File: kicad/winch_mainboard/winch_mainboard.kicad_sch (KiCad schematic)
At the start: 35 parts, among them J1 PWR_IN_24V (from Victron 96V-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, J10 Heltec WiFi LoRa 32 V4 - Head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, J11 Heltec WiFi LoRa 32 V4 - Head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, J12 Hall sensors (drum direction), J2 CAN_BUS (to Fardriver), J3 To GIGA UART (TXD,RXD,GND), J4 HX711 module (3V3,GND,DT,SCK), J6 Spare I/O, J7 Line cut switch (winch), J8 Winchman remote switches, J9 Cut motor out (24V) - A/B = K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, K1 Relay 24V coil (Songle SRD-24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, Q1 BC337-40, U1 ESP32-S3 N16R8 DevKitC-1, U3 SN65HVD230

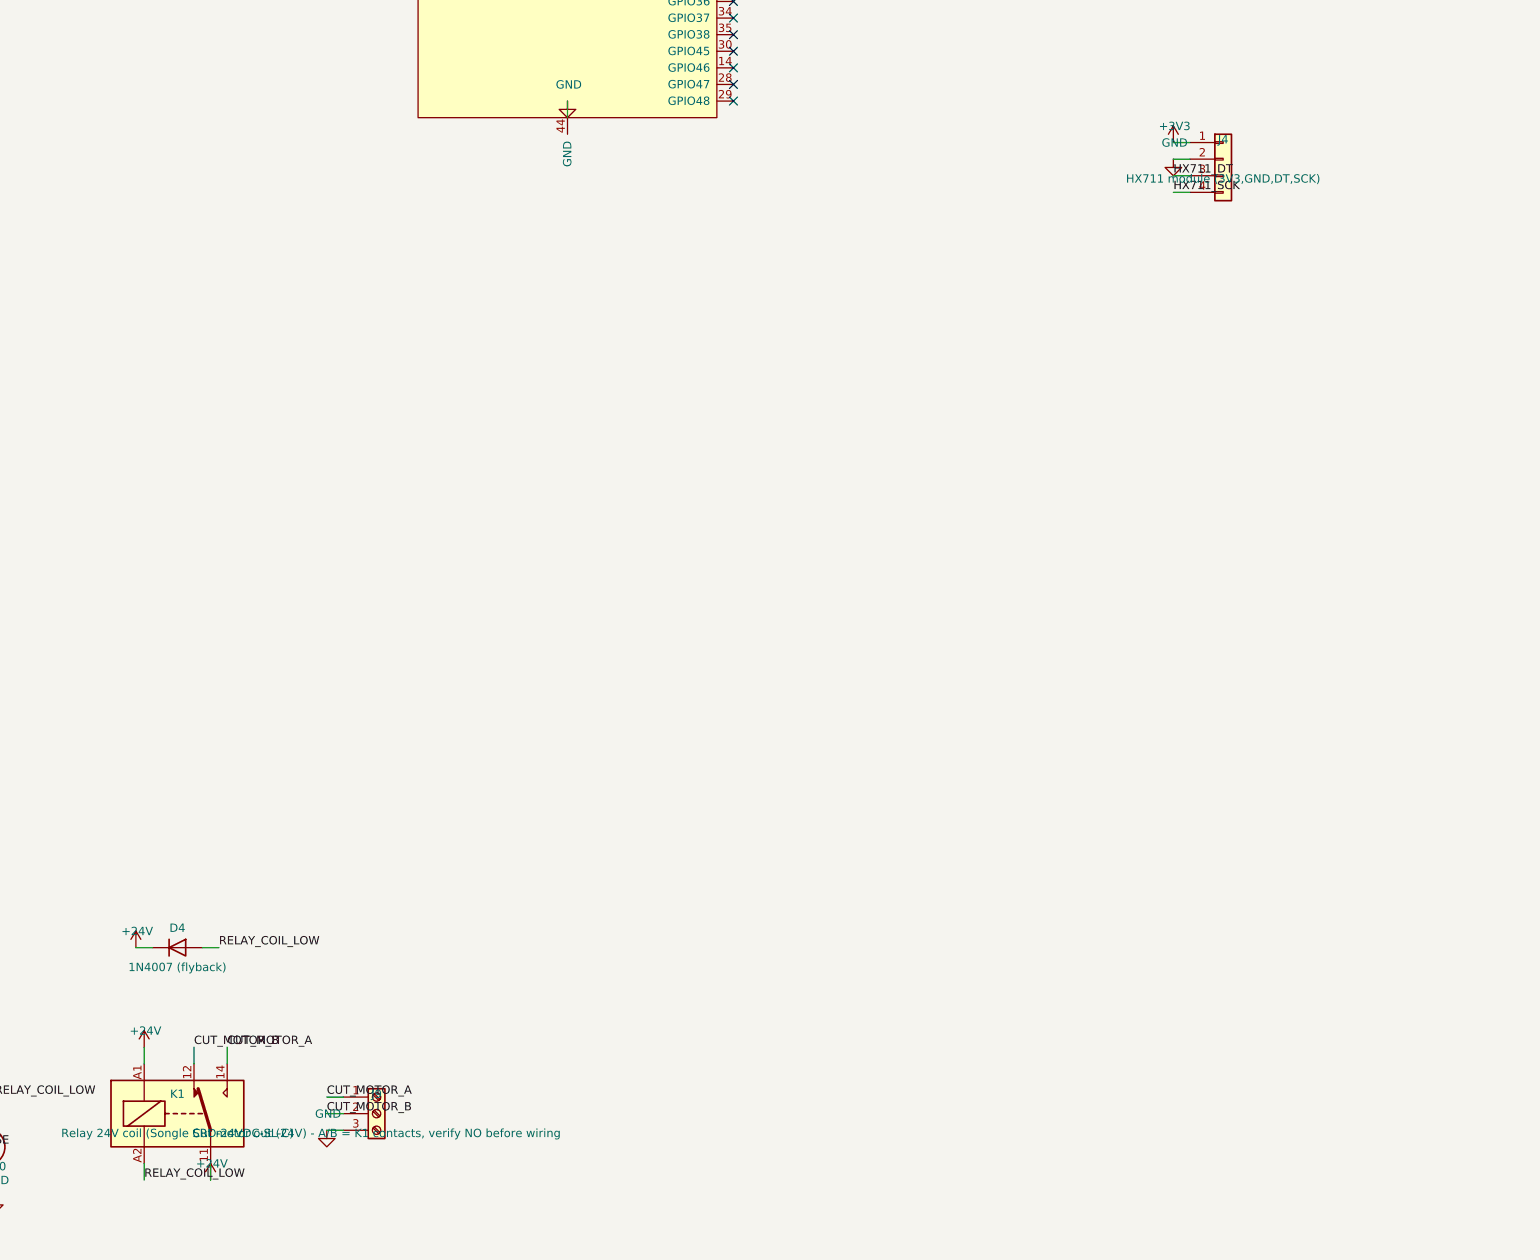
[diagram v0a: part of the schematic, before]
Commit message: update
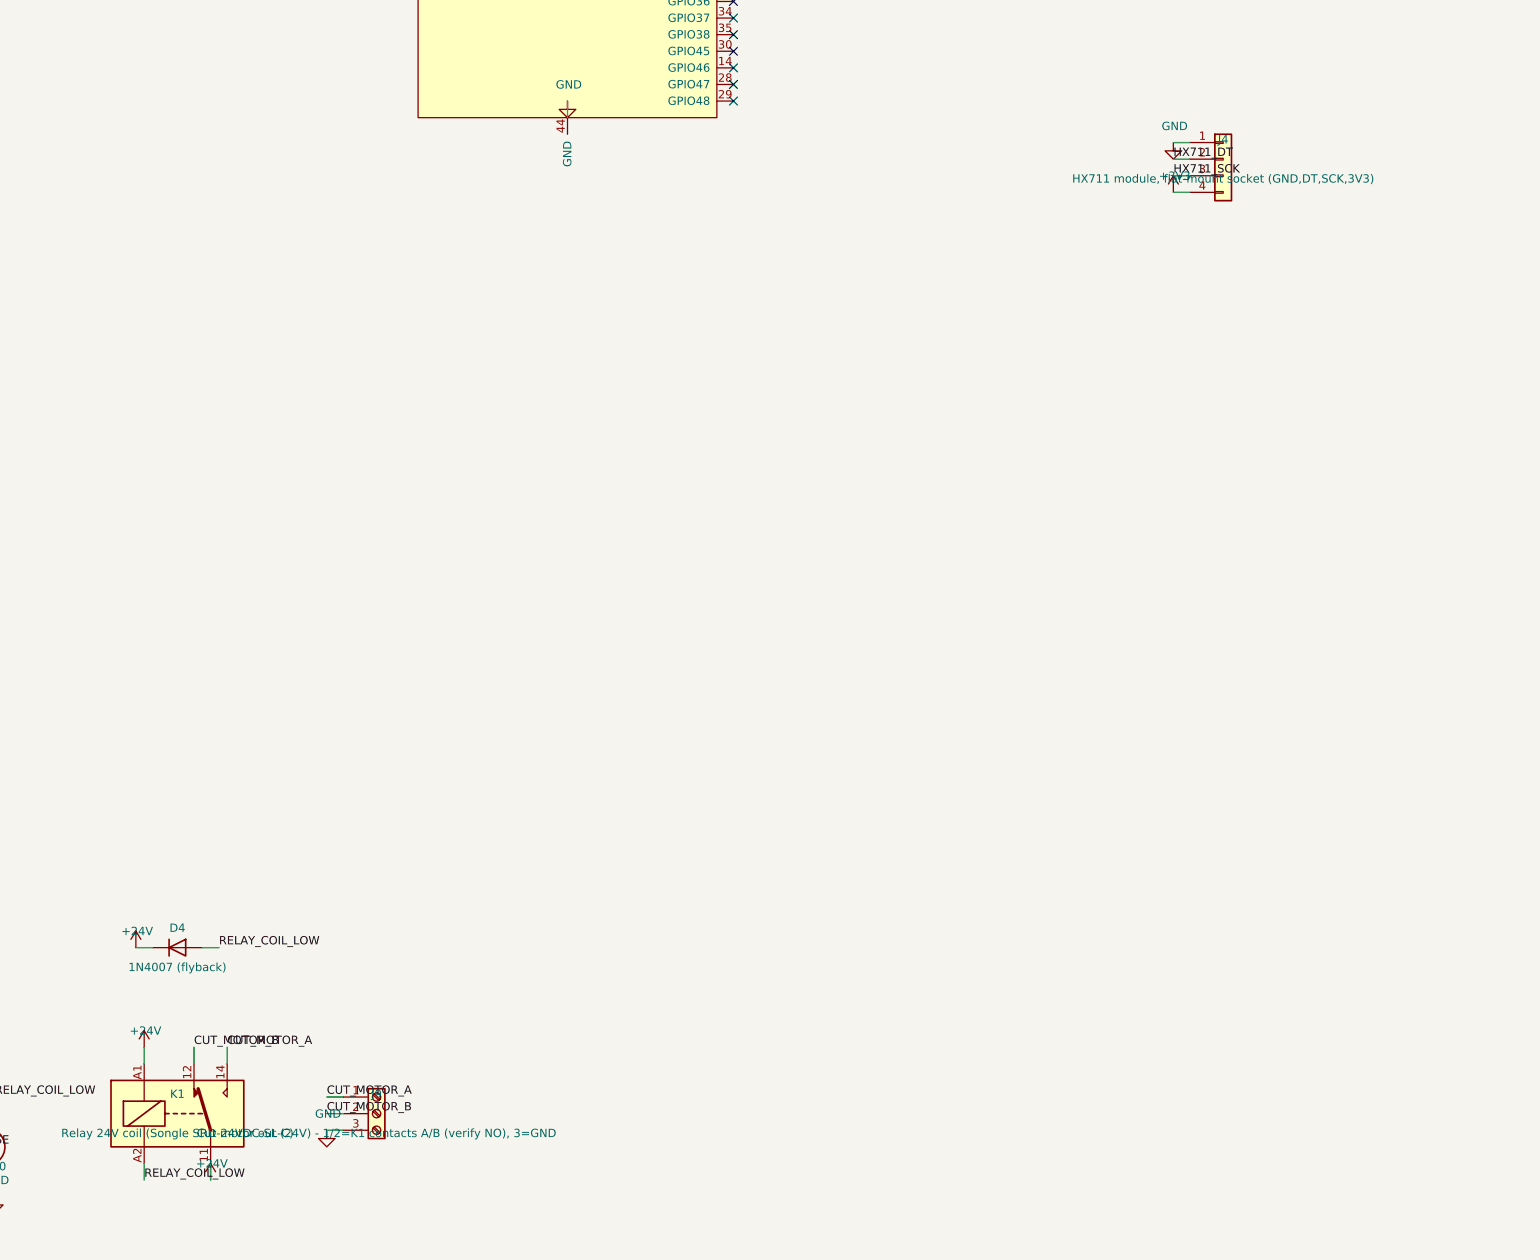
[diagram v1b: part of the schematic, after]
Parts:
- J4: value HX711 module (3V3,GND,DT,SCK) -> HX711 module, flat-mount socket (GND,DT,SCK,3V3); footprint Connector_JST:JST_XH_B4B-XH-A_1x04_P2.50mm_Vertical -> Connector_PinSocket_2.54mm:PinSocket_1x04_P2.54mm_Vertical
- J9: value Cut motor out (24V) - A/B = K1 contacts, verify NO before wiring -> Cut motor out (24V) - 1/2=K1 contacts A/B (verify NO), 3=GND
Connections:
- net +3V3: now also J4.4 (Pin_4); no longer J4.1 (Pin_1)
- net GND: now also J4.1 (Pin_1); no longer J4.2 (Pin_2)
- net HX711_DT: now also J4.2 (Pin_2); no longer J4.3 (Pin_3)
- net HX711_SCK: now also J4.3 (Pin_3); no longer J4.4 (Pin_4)
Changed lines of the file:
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@@
 	)
 	(label "HX711_DT"
-		(at 312.42 201.93 0)
+		(at 312.42 199.39 0)
 		(effects
 			(font
@@
 	)
 	(label "HX711_SCK"
-		(at 312.42 204.47 0)
+		(at 312.42 201.93 0)
 		(effects
 			(font
@@
 	(symbol
 		(lib_id "power:+3V3")
-		(at 312.42 196.85 0)
+		(at 312.42 204.47 0)
 		(unit 1)
 		(exclude_from_sim no)
@@
 		(dnp no)
 		(property "Reference" "#PWR026"
-			(at 312.42 199.85 0)
+			(at 312.42 207.47 0)
 			(hide yes)
 			(effects
@@
 		)
 		(property "Value" "+3V3"
-			(at 312.62 194.35 0)
+			(at 312.62 201.97 0)
 			(effects
 				(font
@@
 		)
 		(property "Footprint" ""
-			(at 312.42 196.85 0)
+			(at 312.42 204.47 0)
 			(hide yes)
 			(effects
@@
 		)
 		(property "Datasheet" ""
-			(at 312.42 196.85 0)
+			(at 312.42 204.47 0)
 			(hide yes)
 			(effects
@@
 	(symbol
 		(lib_id "power:GND")
-		(at 312.42 199.39 0)
+		(at 312.42 196.85 0)
 		(unit 1)
 		(exclude_from_sim no)
@@
 		(dnp no)
 		(property "Reference" "#PWR027"
-			(at 312.42 202.39 0)
+			(at 312.42 199.85 0)
 			(hide yes)
 			(effects
@@
 		)
 		(property "Value" "GND"
-			(at 312.62 196.89 0)
+			(at 312.62 194.35 0)
 			(effects
 				(font
@@
 		)
 		(property "Footprint" ""
-			(at 312.42 199.39 0)
+			(at 312.42 196.85 0)
 			(hide yes)
 			(effects
@@
 		)
 		(property "Datasheet" ""
-			(at 312.42 199.39 0)
+			(at 312.42 196.85 0)
 			(hide yes)
 			(effects
@@
 			)
 		)
-		(property "Value" "HX711 module (3V3,GND,DT,SCK)"
+		(property "Value" "HX711 module, flat-mount socket (GND,DT,SCK,3V3)"
 			(at 320.04 202.39 0)
 			(effects
@@
 			)
 		)
-		(property "Footprint" "Connector_JST:JST_XH_B4B-XH-A_1x04_P2.50mm_Vertical"
+		(property "Footprint" "Connector_PinSocket_2.54mm:PinSocket_1x04_P2.54mm_Vertical"
 			(at 320.04 199.39 0)
 			(hide yes)
@@
 			)
 		)
-		(property "Value" "Cut motor out (24V) - A/B = K1 contacts, verify NO before wiring"
+		(property "Value" "Cut motor out (24V) - 1/2=K1 contacts A/B (verify NO), 3=GND"
 			(at 190.5 348.44 0)
 			(effects
